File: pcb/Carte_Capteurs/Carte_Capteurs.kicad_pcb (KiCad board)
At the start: 2 copper layers, 129.9 x 60 mm, 17 parts, among them J10 Conn_01x05, J11 Conn_01x04, J12 Conn_01x04, J5 Conn_02x07_Odd_Even, J6 Molex KK 254, J7 Samtec FTS-105-01-L-DV, J8 Samtec FTS-105-01-L-DV, J9 Conn_01x05, U1 FRDM-KL25Z, U2 XBee

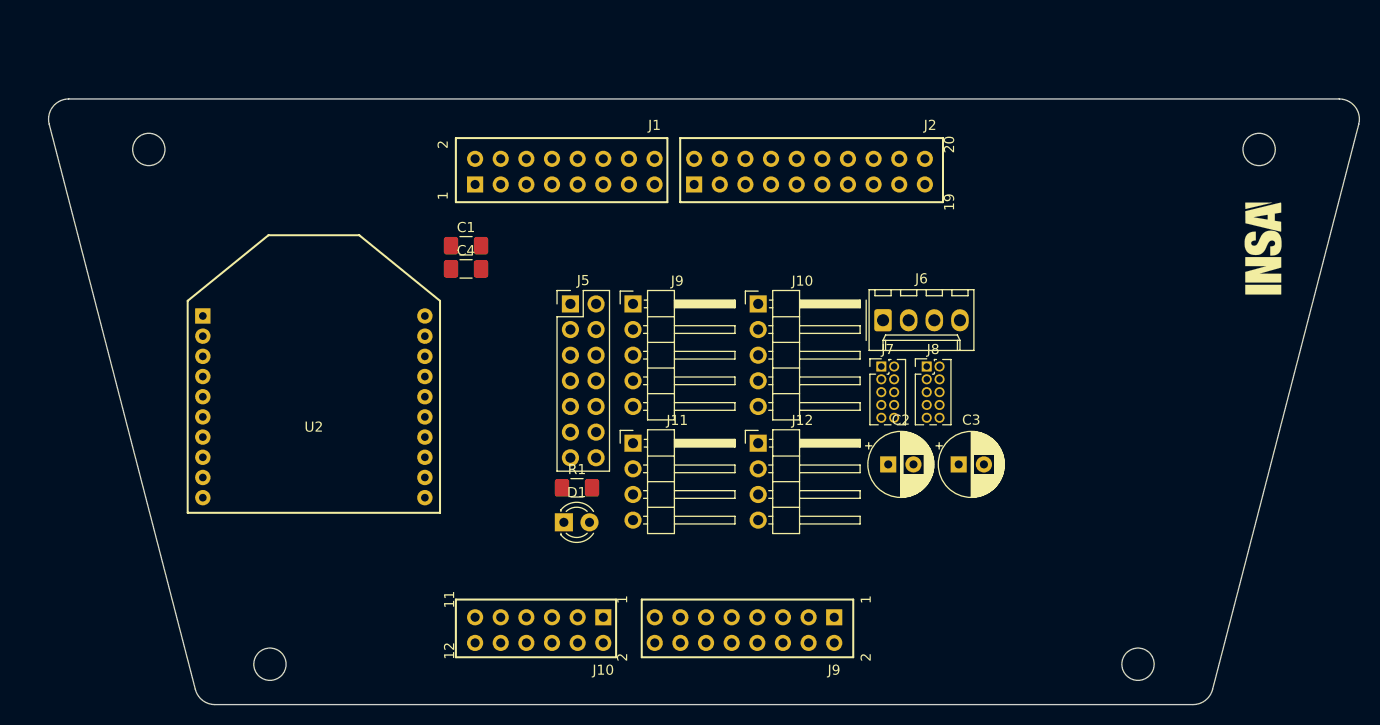
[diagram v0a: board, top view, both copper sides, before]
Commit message: sauvegarde intermediaire
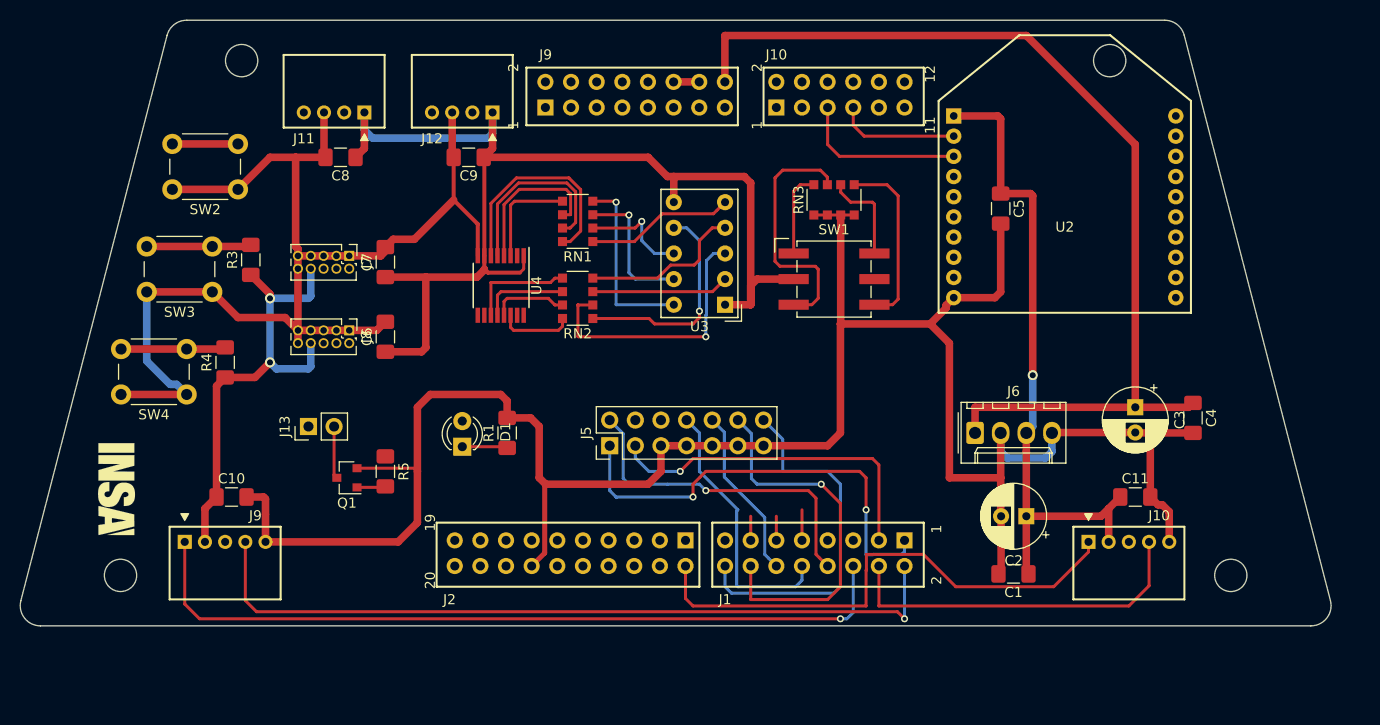
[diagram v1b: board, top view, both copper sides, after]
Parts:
- added C10: 100nF, Capacitor_SMD:C_1206_3216Metric_Pad1.42x1.75mm_HandSolder, F.Cu at (108.0, 113.7)
- added C11: 100nF, Capacitor_SMD:C_1206_3216Metric_Pad1.42x1.75mm_HandSolder, F.Cu at (197.5, 113.7)
- added C5: 100nF, Capacitor_SMD:C_1206_3216Metric_Pad1.42x1.75mm_HandSolder, F.Cu at (184.2, 85.1)
- added C6: 100nF, Capacitor_SMD:C_1206_3216Metric_Pad1.42x1.75mm_HandSolder, F.Cu at (123.2, 97.8)
- added C7: 100nF, Capacitor_SMD:C_1206_3216Metric_Pad1.42x1.75mm_HandSolder, F.Cu at (123.2, 90.4)
- added C8: 100nF, Capacitor_SMD:C_1206_3216Metric_Pad1.42x1.75mm_HandSolder, F.Cu at (118.7, 80.0)
- added C9: 100nF, Capacitor_SMD:C_1206_3216Metric_Pad1.42x1.75mm_HandSolder, F.Cu at (131.4, 80.0)
- added J13: Conn_01x02, Connector_PinHeader_2.54mm:PinHeader_1x02_P2.54mm_Vertical, F.Cu at (115.6, 106.7)
- added Q1: NTR3C21NZT1G, Package_TO_SOT_SMD:SOT-23, F.Cu at (119.4, 111.8)
- added R3: 10K, Resistor_SMD:R_1206_3216Metric_Pad1.42x1.75mm_HandSolder, F.Cu at (109.9, 90.2)
- added R4: 10K, Resistor_SMD:R_1206_3216Metric_Pad1.42x1.75mm_HandSolder, F.Cu at (107.3, 100.3)
- added R5: 100R, Resistor_SMD:R_1206_3216Metric_Pad1.42x1.75mm_HandSolder, F.Cu at (123.2, 111.1)
- added RN1: 100R, Resistor_SMD:R_Array_Convex_4x1206, F.Cu at (142.2, 86.4)
- added RN2: 100R, Resistor_SMD:R_Array_Convex_4x1206, F.Cu at (142.2, 94.0)
- added RN3: 10K, Resistor_SMD:R_Array_Convex_4x1206, F.Cu at (167.6, 84.2)
- added SW1: SMR8016C-1, Insa:Nidec_Copal_SMR-8016C, F.Cu at (167.6, 92.1)
- added SW2: Reset, Button_Switch_THT:SW_PUSH_6mm_H4.3mm, F.Cu at (108.6, 83.2)
- added SW3: USER1, Button_Switch_THT:SW_PUSH_6mm_H4.3mm, F.Cu at (106.0, 93.3)
- added SW4: USER2, Button_Switch_THT:SW_PUSH_6mm_H4.3mm, F.Cu at (103.5, 103.5)
- added U3: HDSP-7501, Display_7Segment:HDSP-A151, F.Cu at (156.8, 94.6)
- added U4: TCL6C598, Package_SO:TSSOP-16_4.4x5mm_P0.65mm, F.Cu at (134.6, 92.7)
- J10, J9: value Conn_01x05 -> DF3A-5P-2DS; footprint Connector_PinHeader_2.54mm:PinHeader_1x05_P2.54mm_Horizontal -> Insa:DF3A-5P-2DS
- J11, J12: value Conn_01x04 -> DF3A-4P-2DS; footprint Connector_PinHeader_2.54mm:PinHeader_1x04_P2.54mm_Horizontal -> Insa:DF3A-4P-2DS
- moved Logo1 116.4 mm to (96.4, 113.0), turned to 270 degrees
- moved U2 77.0 mm to (190.5, 81.9)
- moved C4 73.5 mm to (203.2, 105.8), turned to 270 degrees
- moved C1 63.2 mm to (185.4, 121.3), turned to 180 degrees
- moved J8 57.3 mm to (119.6, 97.2), turned to 270 degrees
- moved J7 53.8 mm to (119.6, 89.8), turned to 270 degrees
- moved J9 46.8 mm to (107.3, 118.1)
- moved J11 44.2 mm to (118.1, 75.6), turned to 180 degrees
- moved J12 44.0 mm to (130.8, 75.6), turned to 180 degrees
- moved J10 43.6 mm to (196.8, 118.1)
- moved C3 18.4 mm to (197.5, 104.8), turned to 270 degrees
- moved C2 14.6 mm to (186.7, 115.6), turned to 180 degrees
- moved J5 14.6 mm to (145.4, 108.6), turned to 90 degrees
- moved J6 14.4 mm to (181.6, 107.3)
- moved D1 12.5 mm to (130.8, 108.7), turned to 90 degrees
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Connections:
- J10 pad 1: (no net) -> /ENC_INDEX2
- J10 pad 2: (no net) -> +3V3
- J10 pad 3: (no net) -> /ENC_SIG_A2
- J10 pad 4: (no net) -> /ENC_SIG_B2
- J10 pad 5: (no net) -> GND
- J11 pad 1: (no net) -> +3V3
- J11 pad 2: (no net) -> /SENS_SDA1
- J11 pad 3: (no net) -> GND
- J11 pad 4: (no net) -> /SENS_SCL1
- J12 pad 1: (no net) -> +3V3
- J12 pad 2: (no net) -> /SENS_SDA2
- J12 pad 3: (no net) -> GND
- J12 pad 4: (no net) -> /SENS_SCL2
- J5 pad 1: (no net) -> /DISABLE_MOT_R
- J5 pad 10: (no net) -> /PWM_MOT_R_2
- J5 pad 12: (no net) -> /PWM_MOT_L_1
- J5 pad 14: (no net) -> /PWM_MOT_L_2
- J5 pad 2: (no net) -> /SERVO_PWM
- J5 pad 3: (no net) -> /DISABLE_MOT_L
- J5 pad 4: (no net) -> /FEEDBACK_MOT_R
- J5 pad 6: (no net) -> /FEEDBACK_MOT_L
- J5 pad 8: (no net) -> /PWM_MOT_R_1
- J7 pad 1: (no net) -> GND
- J7 pad 10: (no net) -> GND
- J7 pad 2: (no net) -> /CCD_AD0
- J7 pad 3: (no net) -> GND
- J7 pad 4: (no net) -> /CCD_SI0
- J7 pad 5: (no net) -> GND
- J7 pad 6: (no net) -> /CCD_CLK0
- J7 pad 7: (no net) -> GND
- J7 pad 8: (no net) -> +3V3
- J7 pad 9: (no net) -> GND
- J8 pad 1: (no net) -> GND
- J8 pad 10: (no net) -> GND
- J8 pad 2: (no net) -> /CCD_AD1
- J8 pad 3: (no net) -> GND
- J8 pad 4: (no net) -> /CCD_SI1
- J8 pad 5: (no net) -> GND
- J8 pad 6: (no net) -> /CCD_CLK1
- J8 pad 7: (no net) -> GND
- J8 pad 8: (no net) -> +3V3
- J8 pad 9: (no net) -> GND
- J9 pad 1: (no net) -> /ENC_INDEX1
- J9 pad 2: (no net) -> +3V3
- J9 pad 3: (no net) -> /ENC_SIG_A1
- J9 pad 4: (no net) -> /ENC_SIG_B1
- J9 pad 5: (no net) -> GND
- U1 pad 1.1: (no net) -> /DISABLE_MOT_R
- U1 pad 1.10: (no net) -> /PWM_MOT_R_1
- U1 pad 1.11: (no net) -> /DISP_SIN
- U1 pad 1.12: (no net) -> /PWM_MOT_R_2
- U1 pad 1.13: (no net) -> /DISP_LATCH
- U1 pad 1.14: (no net) -> /PWM_MOT_L_1
- U1 pad 1.16: (no net) -> /PWM_MOT_L_2
- U1 pad 1.2: (no net) -> /ENC_SIG_B1
- U1 pad 1.3: (no net) -> /DISABLE_MOT_L
- U1 pad 1.4: (no net) -> /ENC_SIG_B2
- U1 pad 1.6: (no net) -> /ENC_INDEX1
- U1 pad 1.8: (no net) -> /SERVO_PWM
- U1 pad 1.9: (no net) -> /DISP_CLK
- U1 pad 2.1: (no net) -> /CAM_LED
- U1 pad 2.10: (no net) -> /SW_USER1
- U1 pad 2.12: (no net) -> /SW_USER2
- U1 pad 2.14: (no net) -> GND
- U1 pad 2.17: (no net) -> /FEEDBACK_MOT_L
- U1 pad 2.18: (no net) -> /SENS_SCL1
- U1 pad 2.2: (no net) -> /ENC_INDEX2
- U1 pad 2.20: (no net) -> /SENS_SDA1
- U1 pad 2.4: (no net) -> /FEEDBACK_MOT_R
- U1 pad 3.1: (no net) -> /CCD_SI0
- U1 pad 3.11: (no net) -> /ROT_SW_2
- U1 pad 3.12: (no net) -> GND
- U1 pad 3.13: (no net) -> /ROT_SW_4
- U1 pad 3.14: (no net) -> GND
- U1 pad 3.15: (no net) -> /ROT_SW_8
- U1 pad 3.3: (no net) -> /CCD_CLK0
- U1 pad 3.5: (no net) -> /CCD_SI1
- U1 pad 3.6: (no net) -> /RESET
- U1 pad 3.7: (no net) -> /CCD_CLK1
- U1 pad 3.9: (no net) -> /ROT_SW_1
- U1 pad 4.10: (no net) -> /CCD_AD0
- U1 pad 4.12: (no net) -> /CCD_AD1
- U1 pad 4.2: (no net) -> /SENS_SCL2
- U1 pad 4.4: (no net) -> /SENS_SDA2
- U1 pad 4.5: (no net) -> /USART_TX
- U1 pad 4.6: (no net) -> /ENC_SIG_A1
- U1 pad 4.7: (no net) -> /USART_RX
- U1 pad 4.8: (no net) -> /ENC_SIG_A2
- U2 pad 2: (no net) -> /USART_RX
- U2 pad 3: (no net) -> /USART_TX
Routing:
- net GND: track 0.00 -> 341.3 mm
- net +3V3: track 0.00 -> 227.5 mm, vias 0 -> 3
- net +BATT: track 0.00 -> 100.1 mm
- net /ENC_INDEX1: track 0.00 -> 77.9 mm, vias 0 -> 1
- net /ENC_SIG_B1: track 0.00 -> 77.1 mm, vias 0 -> 1
- net /ENC_INDEX2: track 0.00 -> 52.3 mm
- net /DISABLE_MOT_R: track 0.00 -> 44.9 mm, vias 0 -> 2
- net /PWM_MOT_L_1: track 0.00 -> 37.3 mm, vias 0 -> 1
- net /PWM_MOT_L_2: track 0.00 -> 36.3 mm
- net /ENC_SIG_B2: track 0.00 -> 35.9 mm
- net /DISABLE_MOT_L: track 0.00 -> 34.1 mm, vias 0 -> 1
- net /SERVO_PWM: track 0.00 -> 33.4 mm, vias 0 -> 1
- net Net-(RN2-Pad2): track 0.00 -> 27.0 mm, vias 0 -> 1
- net /PWM_MOT_R_1: track 0.00 -> 26.7 mm
- net /ROT_SW_2: track 0.00 -> 25.0 mm
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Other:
- outline, holes or cut-outs redrawn
- net class Default: trace_width 0.25 -> 0.35; via_dia 0.8 -> 0.7
- net class Power added: clearance 0.2, trace_width 0.5, via_dia 1, via_drill 0.6
